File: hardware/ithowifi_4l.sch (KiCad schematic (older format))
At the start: 31 parts, among them J1 CONN_01X07, J2 conn, J3 Conn_Coaxial, J4 TC2030-MCP-NL, J5 Conn_02x02_Odd_Even, Q1 BSS138, Q2 BSS138, SW1 Fail safe, U1 ESP32-WROOM, U2 CC1101-868MHz-Module

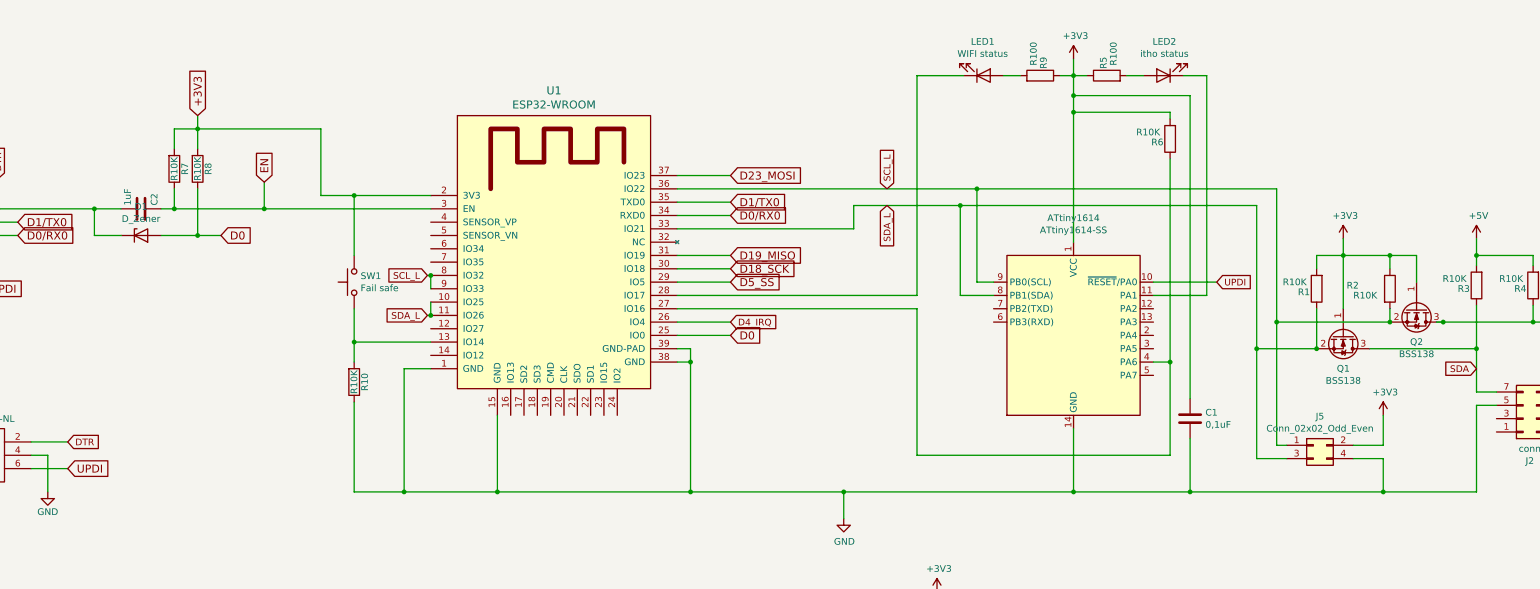
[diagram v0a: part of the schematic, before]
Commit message: Update hardware files
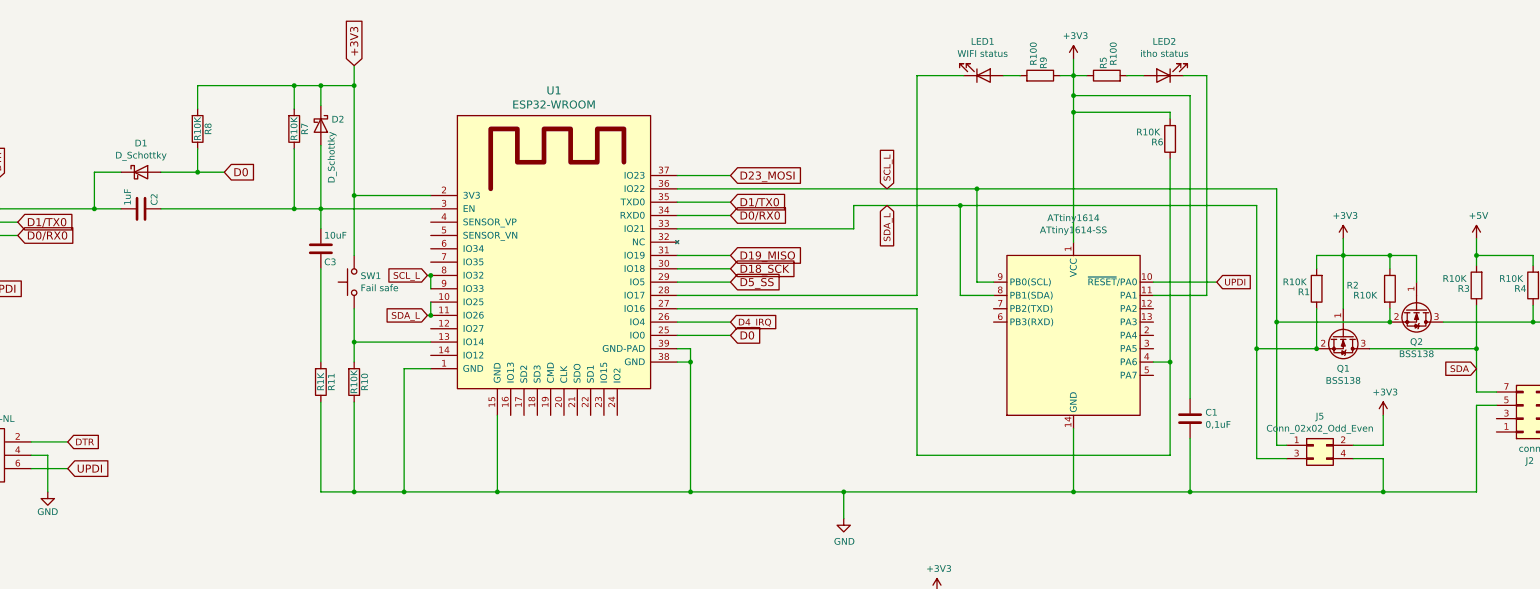
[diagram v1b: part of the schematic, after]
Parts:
- removed D1: D_Zener, Diode_SMD:D_SOD-123, symbol Device:D_Zener
- added C3: 10uF, Capacitor_SMD:C_0805_2012Metric, symbol Device:C
- added D1, D2: D_Schottky, Diode_SMD:D_SOD-123, symbol Device:D_Schottky
- added R11: R1K, Resistor_SMD:R_0805_2012Metric, symbol Device:R
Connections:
- net +3V3: now also D2.1 (K)
- net D0: now also D1.2 (A)
- net DTR: now also D1.1 (K)
- net GND: now also R11.1
- net EN: no longer names the net of C2.1, R7.1, U1.3 (EN)
- net EN: now also C3.2, D2.2 (A)
- new net: C3.1, R11.2
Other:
- moved on the sheet: R7, R8
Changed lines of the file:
@@
 	12825 4150 13625 4150
-Wire Wire Line
-	13325 3950 13375 3950
 Wire Wire Line
 	12625 3325 12625 3450
@@
 	13625 3825 13625 4150
 Connection ~ 13625 4150
-Connection ~ 13375 3950
 Wire Wire Line
 	13375 3950 14050 3950
@@
 	-1   0    0    -1
 $EndComp
-$Comp
-L Device:C C?
-U 1 1 5FBF50D4
-P 3600 3100
-AR Path="/5FAE7423/5FBF50D4" Ref="C?"  Part="1"
-AR Path="/5FBF50D4" Ref="C2"  Part="1"
-F 0 "C2" H 3625 3200 50  0000 L CNN
-F 1 "1uF" H 3625 3000 50  0000 L CNN
-F 2 "Capacitor_SMD:C_0805_2012Metric" H 3638 2950 50  0001 C CNN
-F 3 "" H 3600 3100 50  0001 C CNN
-F 4 "C28323" H 3600 3100 50  0001 C CNN "LCSC"
-	1    3600 3100
-	0    1    -1   0
-$EndComp
 Text GLabel 2675 3200 2    60   Input ~ 0
 D1/TX0
-Text GLabel 2675 3300 2    60   Input ~ 0
-D0/RX0
 NoConn ~ 2125 3500
 $Comp
@@
 	-1   0    0    -1
 $EndComp
-$Comp
-L Device:R R?
-U 1 1 5FBF50E3
-P 4025 2800
-AR Path="/5FAE7423/5FBF50E3" Ref="R?"  Part="1"
-AR Path="/5FBF50E3" Ref="R8"  Part="1"
-F 0 "R8" V 4105 2800 50  0000 C CNN
-F 1 "R10K" V 4025 2800 50  0000 C CNN
-F 2 "Resistor_SMD:R_0805_2012Metric" V 3955 2800 50  0001 C CNN
-F 3 "" H 4025 2800 50  0001 C CNN
-F 4 "C17414" H 4025 2800 50  0001 C CNN "LCSC"
-	1    4025 2800
-	1    0    0    1
-$EndComp
-Text GLabel 4200 3300 2    60   Input ~ 0
-D0
-Text GLabel 4025 2400 1    60   Input ~ 0
+Text GLabel 5200 2025 1    60   Input ~ 0
 +3V3
 Text GLabel 2225 2875 1    60   Input ~ 0
@@
 	2125 3200 2675 3200
 Wire Wire Line
-	3850 2950 3850 3100
-Connection ~ 3850 3100
-Wire Wire Line
-	3850 2650 3850 2500
-Wire Wire Line
-	3850 2500 4025 2500
-Connection ~ 4025 2500
-Wire Wire Line
-	4025 2400 4025 2500
+	5200 2025 5200 2175
 Wire Wire Line
 	2225 3400 2225 2875
-Wire Wire Line
-	4025 2500 4025 2650
 $Comp
 L nrg_watch:ESP32-WROOM U?
@@
 D4_IRQ
 Wire Wire Line
-	3750 3100 3850 3100
-Wire Wire Line
-	4950 2500 4950 3000
-Wire Wire Line
-	4200 3300 4025 3300
-$Comp
-L Device:D_Zener D?
-U 1 1 5FBF5174
-P 3600 3300
-AR Path="/5FAE7423/5FBF5174" Ref="D?"  Part="1"
-AR Path="/5FBF5174" Ref="D1"  Part="1"
-F 0 "D1" H 3600 3516 50  0000 C CNN
-F 1 "D_Zener" H 3600 3425 50  0000 C CNN
-F 2 "Diode_SMD:D_SOD-123" H 3600 3300 50  0001 C CNN
-F 3 "~" H 3600 3300 50  0001 C CNN
-F 4 "C8598" H 3600 3300 50  0001 C CNN "LCSC"
-	1    3600 3300
-	1    0    0    -1
-$EndComp
-Wire Wire Line
-	3750 3300 4025 3300
-Connection ~ 4025 3300
-Wire Wire Line
 	2125 3100 2525 3100
-Wire Wire Line
-	3450 3300 3250 3300
-Wire Wire Line
-	3250 3300 3250 3100
-Connection ~ 3250 3100
-Wire Wire Line
-	3250 3100 3450 3100
-Wire Wire Line
-	4025 2950 4025 3300
 Text GLabel 2400 3700 2    60   Input ~ 0
 UPDI
@@
 Wire Wire Line
 	10600 2375 10600 3350
-Wire Wire Line
-	4025 2500 4950 2500
-Wire Wire Line
-	3850 3100 4525 3100
-Wire Wire Line
-	4525 2900 4525 3100
-Connection ~ 4525 3100
 Wire Wire Line
 	8150 6800 8475 6800
@@
 Wire Wire Line
 	3750 6550 4175 6550
-Wire Wire Line
-	4950 3000 5200 3000
 Wire Wire Line
 	4475 7425 4475 7225
@@
 	5200 4100 5200 4250
 Connection ~ 5200 4100
-Connection ~ 5200 3000
 Wire Wire Line
 	5200 3000 5775 3000
-Text GLabel 4525 2900 1    60   Input ~ 0
-EN
 Wire Wire Line
 	7725 5225 8875 5225
-Wire Wire Line
-	4525 3100 5775 3100
 Text GLabel 3050 5050 2    60   Input ~ 0
 UPDI
@@
 	2525 2875 2525 3100
 Connection ~ 2525 3100
-Wire Wire Line
-	2525 3100 3250 3100
 Text GLabel 3050 4850 2    50   Input ~ 0
 DTR
@@
 	14275 4775 14975 4775
 $Comp
+L Device:C C?
+U 1 1 5FBF50D4
+P 3600 3100
+AR Path="/5FAE7423/5FBF50D4" Ref="C?"  Part="1"
+AR Path="/5FBF50D4" Ref="C2"  Part="1"
+F 0 "C2" H 3625 3200 50  0000 L CNN
+F 1 "1uF" H 3625 3000 50  0000 L CNN
+F 2 "Capacitor_SMD:C_0805_2012Metric" H 3638 2950 50  0001 C CNN
+F 3 "" H 3600 3100 50  0001 C CNN
+F 4 "C28323" H 3600 3100 50  0001 C CNN "LCSC"
+	1    3600 3100
+	0    1    -1   0
+$EndComp
+Connection ~ 5200 2175
+$Comp
+L Device:R R?
+U 1 1 5FBF50E3
+P 4025 2500
+AR Path="/5FAE7423/5FBF50E3" Ref="R?"  Part="1"
+AR Path="/5FBF50E3" Ref="R8"  Part="1"
+F 0 "R8" V 4105 2500 50  0000 C CNN
+F 1 "R10K" V 4025 2500 50  0000 C CNN
+F 2 "Resistor_SMD:R_0805_2012Metric" V 3955 2500 50  0001 C CNN
+F 3 "" H 4025 2500 50  0001 C CNN
+F 4 "C17414" H 4025 2500 50  0001 C CNN "LCSC"
+	1    4025 2500
+	1    0    0    1
+$EndComp
+$Comp
+L Device:C C?
+U 1 1 612C4FB5
+P 4950 3400
+AR Path="/5FAE7423/612C4FB5" Ref="C?"  Part="1"
+AR Path="/612C4FB5" Ref="C3"  Part="1"
+F 0 "C3" H 4975 3500 50  0000 L CNN
+F 1 "10uF" H 4975 3300 50  0000 L CNN
+F 2 "Capacitor_SMD:C_0805_2012Metric" H 4988 3250 50  0001 C CNN
+F 3 "" H 4950 3400 50  0001 C CNN
+F 4 "C28323" H 4950 3400 50  0001 C CNN "LCSC"
+	1    4950 3400
+	1    0    0    1
+$EndComp
+Wire Wire Line
+	4950 3250 4950 3100
+Connection ~ 4950 3100
+Wire Wire Line
+	4950 3100 5775 3100
+Wire Wire Line
+	4950 3550 4950 4250
+Wire Wire Line
+	4950 5225 5200 5225
+Connection ~ 5200 5225
+$Comp
+L Device:R R?
+U 1 1 613B5125
+P 4950 4400
+AR Path="/5FAE7423/613B5125" Ref="R?"  Part="1"
+AR Path="/613B5125" Ref="R11"  Part="1"
+F 0 "R11" V 5030 4400 50  0000 C CNN
+F 1 "R1K" V 4950 4400 50  0000 C CNN
+F 2 "Resistor_SMD:R_0805_2012Metric" V 4880 4400 50  0001 C CNN
+F 3 "" H 4950 4400 50  0001 C CNN
+F 4 "C17414" H 4950 4400 50  0001 C CNN "LCSC"
+	1    4950 4400
+	1    0    0    1
+$EndComp
+Wire Wire Line
+	4950 4550 4950 5225
+$Comp
 L Device:R R?
 U 1 1 5FBF50E9
-P 3850 2800
+P 4750 2500
 AR Path="/5FAE7423/5FBF50E9" Ref="R?"  Part="1"
 AR Path="/5FBF50E9" Ref="R7"  Part="1"
-F 0 "R7" V 3930 2800 50  0000 C CNN
-F 1 "R10K" V 3850 2800 50  0000 C CNN
-F 2 "Resistor_SMD:R_0805_2012Metric" V 3780 2800 50  0001 C CNN
-F 3 "" H 3850 2800 50  0001 C CNN
-F 4 "C17414" H 3850 2800 50  0001 C CNN "LCSC"
-	1    3850 2800
+F 0 "R7" V 4830 2500 50  0000 C CNN
+F 1 "R10K" V 4750 2500 50  0000 C CNN
+F 2 "Resistor_SMD:R_0805_2012Metric" V 4680 2500 50  0001 C CNN
+F 3 "" H 4750 2500 50  0001 C CNN
+F 4 "C17414" H 4750 2500 50  0001 C CNN "LCSC"
+	1    4750 2500
 	1    0    0    1
 $EndComp
+Wire Wire Line
+	4950 2625 4950 3100
+Connection ~ 4950 2175
+Wire Wire Line
+	4950 2175 5200 2175
+$Comp
+L Device:D_Schottky D1
+U 1 1 613CE017
+P 3600 2825
+F 0 "D1" H 3600 3042 50  0000 C CNN
+F 1 "D_Schottky" H 3600 2951 50  0000 C CNN
+F 2 "Diode_SMD:D_SOD-123" H 3600 2825 50  0001 C CNN
+F 3 "~" H 3600 2825 50  0001 C CNN
+	1    3600 2825
+	1    0    0    -1
+$EndComp
+Wire Wire Line
+	3250 2825 3450 2825
+Text GLabel 4225 2825 2    60   Input ~ 0
+D0
+Text GLabel 2675 3300 2    60   Input ~ 0
+D0/RX0
+Wire Wire Line
+	2525 3100 3250 3100
+Wire Wire Line
+	3750 2825 4025 2825
+Wire Wire Line
+	3250 2825 3250 3100
+Connection ~ 3250 3100
+Wire Wire Line
+	3250 3100 3450 3100
+Wire Wire Line
+	5200 2175 5200 3000
+Connection ~ 5200 3000
+Wire Wire Line
+	4950 2175 4950 2325
+Wire Wire Line
+	4025 2650 4025 2825
+Connection ~ 4025 2825
+Wire Wire Line
+	4025 2825 4225 2825
+Wire Wire Line
+	4025 2350 4025 2175
+Wire Wire Line
+	4025 2175 4750 2175
+Wire Wire Line
+	3750 3100 4750 3100
+$Comp
+L Device:D_Schottky D2
+U 1 1 6164833C
+P 4950 2475
+F 0 "D2" V 4904 2555 50  0000 L CNN
+F 1 "D_Schottky" H 4995 2555 50  0000 L CNN
+F 2 "Diode_SMD:D_SOD-123" H 4950 2475 50  0001 C CNN
+F 3 "~" H 4950 2475 50  0001 C CNN
+	1    4950 2475
+	0    1    1    0
+$EndComp
+Wire Wire Line
+	4750 2175 4750 2350
+Connection ~ 4750 2175
+Wire Wire Line
+	4750 2175 4950 2175
+Wire Wire Line
+	4750 2650 4750 3100
+Connection ~ 4750 3100
+Wire Wire Line
+	4750 3100 4950 3100
 $EndSCHEMATC
